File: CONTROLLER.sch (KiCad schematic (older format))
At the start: 25 parts, among them J201 Raspberry_Pi_2_3, Q201 BSS138, Q202 BSS138, U201 MCP23017_SO, U202 MAX11616, U203 MAX3232

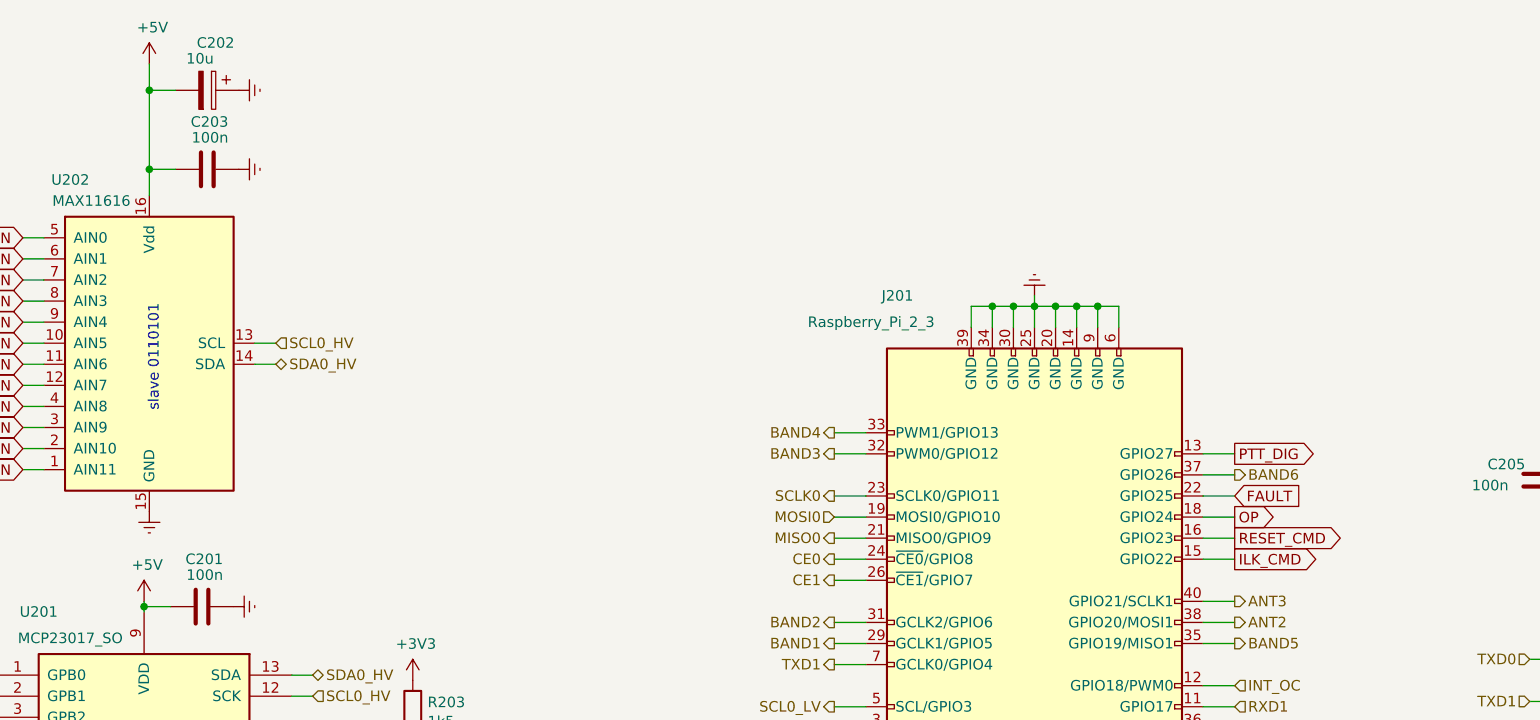
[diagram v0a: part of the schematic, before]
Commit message: Review 1
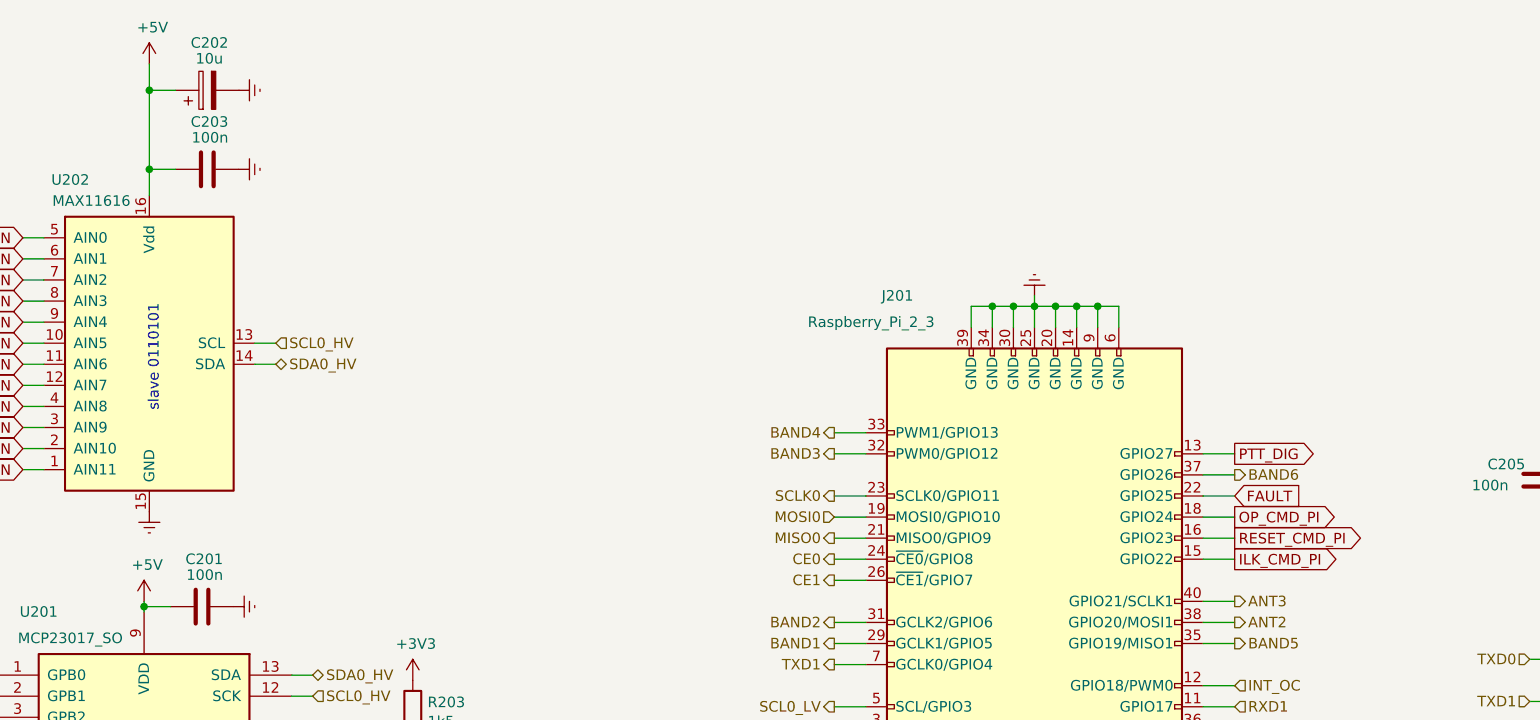
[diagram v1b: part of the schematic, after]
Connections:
- net +5V: now also C202.1; no longer C202.2
- net Earth: now also C202.2; no longer C202.1
- net ILK_CMD renamed ILK_CMD_PI
- net OP renamed OP_CMD_PI
- net RESET_CMD renamed RESET_CMD_PI
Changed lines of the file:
@@
 Sheet 2 4
 Title "RF Amplifier Controller"
-Date "2019-11-23"
+Date "2019-12-01"
 Rev "1"
 Comp "HB9GKW"
@@
 ILK_RF_OL
 Text GLabel 10075 5425 2    50   Output ~ 0
-RESET_CMD
+RESET_CMD_PI
 Text GLabel 3925 7475 0    50   Input ~ 0
 ILK_IDD_OC
@@
 	4925 3675 5050 3675
 Connection ~ 4925 3675
-Wire Wire Line
-	4925 3675 4925 3300
 $Comp
 L power:Earth #PWR?
@@
 	9225 7050 9325 7050
 Text GLabel 10075 5325 2    50   Output ~ 0
-OP
+OP_CMD_PI
 Wire Wire Line
 	10075 5325 9925 5325
 Text GLabel 10075 5525 2    50   Output ~ 0
-ILK_CMD
+ILK_CMD_PI
 Wire Wire Line
 	10075 5525 9925 5525
@@
 AR Path="/5DD09976" Ref="C?"  Part="1"
 AR Path="/5CBD59C6/5DD09976" Ref="C202"  Part="1"
-F 0 "C202" V 4975 3250 50  0000 L CNN
-F 1 "10u" V 5050 3200 50  0000 L CNN
+F 0 "C202" V 5425 3200 50  0000 L CNN
+F 1 "10u" V 5350 3225 50  0000 L CNN
 F 2 "Capacitor_Tantalum_SMD:CP_EIA-6032-28_Kemet-C" H 5238 3150 50  0001 C CNN
 F 3 "~" H 5200 3300 50  0001 C CNN
 	1    5200 3300
-	0    1    1    0
+	0    -1   -1   0
 $EndComp
 $Comp
@@
 	0    -1   -1   0
 $EndComp
-Wire Wire Line
-	5050 3300 4925 3300
-Connection ~ 4925 3300
-Wire Wire Line
-	4925 3300 4925 3175
 Wire Notes Line
 	7925 8050 7925 9825
@@
 	9025 7025 9025 7075
 NoConn ~ 8925 7025
+Wire Wire Line
+	4925 3175 4925 3300
+Wire Wire Line
+	5050 3300 4925 3300
+Connection ~ 4925 3300
+Wire Wire Line
+	4925 3300 4925 3675
 $EndSCHEMATC
